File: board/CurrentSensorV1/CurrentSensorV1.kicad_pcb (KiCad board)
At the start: 2 copper layers, 40.8 x 24.2 mm, 19 parts, among them J1 USB_B_Micro, J2 FTDI_Header, J3 AudioJack3_GroundPinNumbers, J4 0, J5 0, J6 Conn_01x02_Female, J7 Conn_01x02_Female, SW2 SW_SPST_SM_DP, SW3 SW_SPST_SM_DP, U1 UA78M05CDCY, U2 ESP-01v090, U3 ADS1115

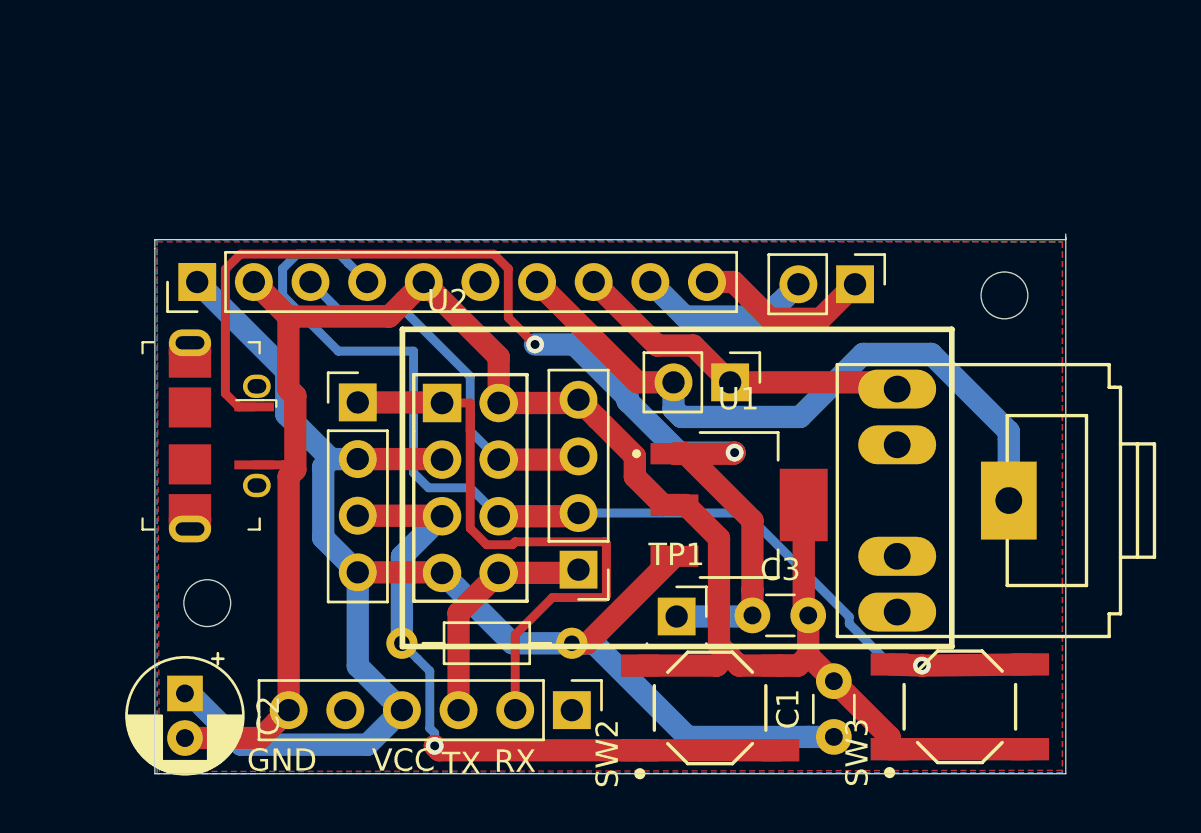
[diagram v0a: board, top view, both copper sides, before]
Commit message: Starting v4
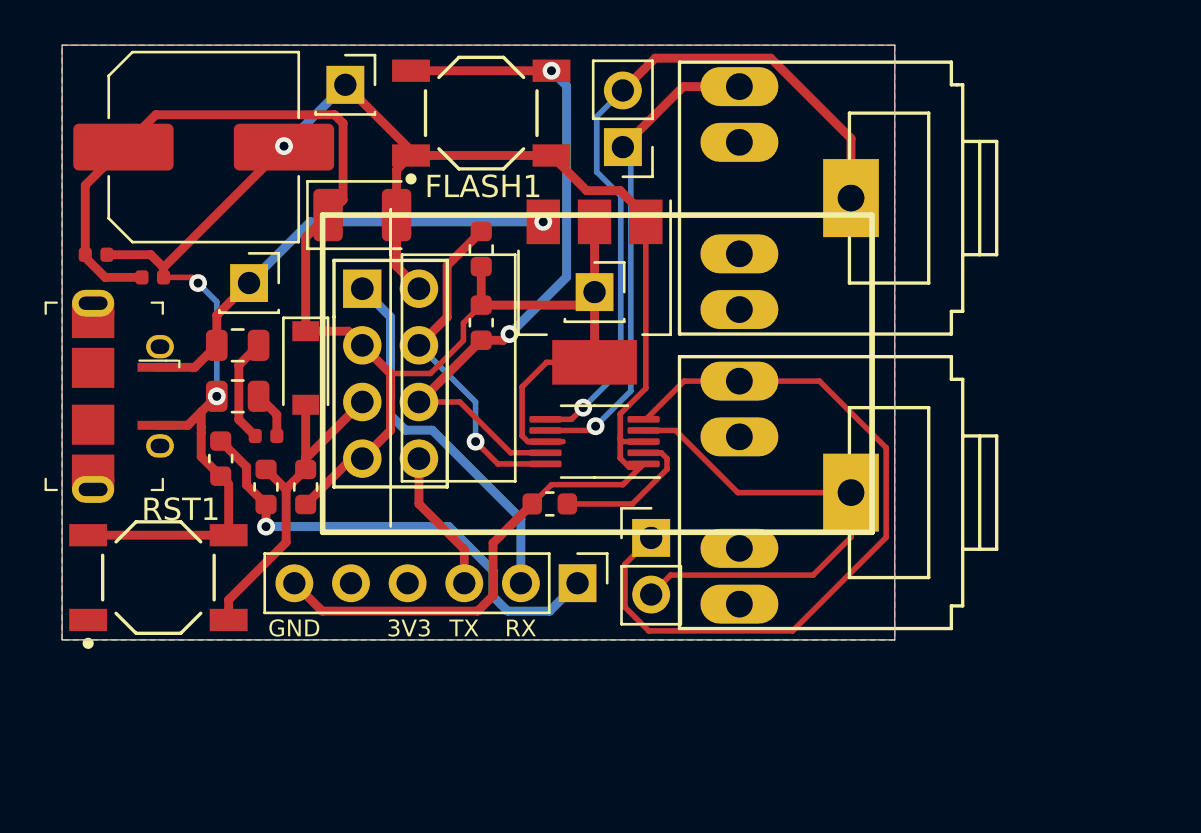
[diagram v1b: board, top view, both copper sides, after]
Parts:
- removed J4, J5: 0, Connector_PinHeader_2.54mm:PinHeader_1x04_P2.54mm_Vertical
- removed R4: R, Resistor_THT:R_Axial_DIN0204_L3.6mm_D1.6mm_P7.62mm_Horizontal
- removed REF** (x2): MountingHole_2.1mm, MountingHole:MountingHole_2.1mm
- added C4: 1000uF, Capacitor_SMD:C_Elec_8x10.2, F.Cu at (139.2, 69.8)
- added C5: 1uF, Capacitor_SMD:C_0402_1005Metric, F.Cu at (136.9, 75.7)
- added C6: 2.2uF, Capacitor_SMD:C_0603_1608Metric, F.Cu at (142.0, 85.1)
- added D1: D, Diode_SMD:D_SOD-123, F.Cu at (143.8, 79.8)
- added FB1: Ferrite_Bead, Resistor_SMD:R_0805_2012Metric, F.Cu at (140.7, 81.0)
- added FB2: Ferrite_Bead, Resistor_SMD:R_0805_2012Metric, F.Cu at (140.7, 78.7)
- added J8: AudioJack3_GroundPinNumbers, audio35mm:Tayda_3.5mm_stereo_TRS_jack_A-853, F.Cu at (166.6, 72.1)
- added R1: 10K, Resistor_SMD:R_0603_1608Metric, F.Cu at (151.6, 74.4)
- added R2: 10K, Resistor_SMD:R_0603_1608Metric, F.Cu at (151.6, 77.7)
- added R3: 10K, Resistor_SMD:R_0603_1608Metric, F.Cu at (154.7, 85.9)
- added R5: 680R, Resistor_SMD:R_0603_1608Metric, F.Cu at (140.0, 83.8)
- added R6: 10K, Resistor_SMD:R_0603_1608Metric, F.Cu at (143.8, 85.1)
- added TP2: TestPoint, Connector_PinSocket_2.54mm:PinSocket_1x01_P2.54mm_Vertical, F.Cu at (156.7, 76.4)
- added TP3: TestPoint, Connector_PinSocket_2.54mm:PinSocket_1x01_P2.54mm_Vertical, F.Cu at (145.5, 67.1)
- C1: value 0.1uF -> 1uF; footprint Capacitor_THT:C_Disc_D3.0mm_W1.6mm_P2.50mm -> Capacitor_SMD:C_0402_1005Metric
- C2: value 470uF -> 100uF; footprint Capacitor_THT:CP_Radial_D5.0mm_P2.00mm -> Capacitor_Tantalum_SMD:CP_EIA-3528-12_Kemet-T
- C3: value 0.33uF -> 1uF; footprint Capacitor_THT:C_Disc_D3.0mm_W1.6mm_P2.50mm -> Capacitor_SMD:C_0402_1005Metric
- TP1: value (none) -> TestPoint
- U1: value UA78M05CDCY -> ADS1015_IC; footprint UA78M05CDCY:SOT230P700X180-4N -> Package_SO:VSSOP-10_3x3mm_P0.5mm
- U3: value ADS1115 -> AMS1117-3.3; footprint Connector_PinHeader_2.54mm:PinHeader_1x10_P2.54mm_Vertical -> Package_TO_SOT_SMD:SOT-223-3_TabPin2
- moved FLASH1 34.2 mm to (151.6, 68.3)
- moved C3 33.6 mm to (134.4, 74.7)
- moved C1 28.8 mm to (142.0, 82.8), turned to 0 degrees
- moved RST1 25.4 mm to (137.2, 89.2)
- moved TP1 24.3 mm to (141.2, 75.9)
- moved C2 22.9 mm to (146.3, 72.9), turned to 0 degrees
- moved U3 17.8 mm to (156.7, 76.4), turned to 270 degrees
- moved J7 12.1 mm to (158.0, 69.8), turned to 180 degrees
- moved J6 7.82 mm to (159.3, 87.4), turned to 0 degrees
- moved J3 7.08 mm to (166.6, 85.3)
- moved U1 7.08 mm to (156.7, 83.1), turned to 180 degrees
- moved U2 6.25 mm to (146.3, 76.2)
- moved J2 5.70 mm to (156.0, 89.4)
- moved J1 4.69 mm to (136.9, 81.0)
- renumbered SW3 to FLASH1, SW2 to RST1
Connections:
- net Net-(J2-Pad2) renamed FTDI_RX
- net Net-(J2-Pad3) renamed FTDI_TX
- net Net-(J5-Pad3) renamed RST
- C1 pad 1: +3V3 -> Net-(C1-Pad1)
- C1 pad 2: GND -> Net-(C1-Pad2)
- C2 pad 2: GND -> ADDR
- C3 pad 1: VBUS -> +3V3
- C3 pad 2: GND -> ADDR
- FLASH1 pad 1: GND -> ADDR
- FLASH1 pad 2: GND -> ADDR
- J1 pad 5: GND -> ADDR
- J2 pad 6: GND -> ADDR
- J3 pad 1: Net-(J3-Pad1) -> AIN0
- J3 pad 3: Net-(J3-Pad3) -> AIN1
- J6 pad 1: Net-(J3-Pad3) -> AIN1
- J6 pad 2: Net-(J3-Pad1) -> AIN0
- J7 pad 1: Net-(J7-Pad1) -> AIN3
- J7 pad 2: Net-(J7-Pad2) -> AIN2
- RST1 pad 3: GND -> ADDR
- RST1 pad 4: GND -> ADDR
- U1 pad 1: VBUS -> ADDR
- U1 pad 2: GND -> /ALERT
- U1 pad 3: +3V3 -> ADDR
- U1 pad 4: GND -> AIN0
- U2 pad 2: GND -> ADDR
- U3 pad 1: +3V3 -> ADDR
- U3 pad 2: GND -> +3V3
- U3 pad 3: SCL -> VBUS
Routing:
- net ADDR: track 0.00 -> 96.3 mm, vias 0 -> 3
- net GND: track 90.6 -> 0.00 mm
- net AIN1: track 0.00 -> 34.3 mm
- net AIN2: track 0.00 -> 32.8 mm, vias 0 -> 1
- net Net-(J3-Pad1): track 30.1 -> 0.00 mm
- net VBUS: track 50.4 -> 22.3 mm, vias 2 -> 1
- net AIN0: track 0.00 -> 22.5 mm
- net AIN3: track 0.00 -> 22.0 mm, vias 0 -> 1
- net Net-(C6-Pad2): track 0.00 -> 21.4 mm, vias 0 -> 1
- net SDA: track 51.1 -> 31.4 mm, vias 1 -> 2
- net Net-(J3-Pad3): track 15.6 -> 0.00 mm
- net RST: track 31.0 -> 16.4 mm, vias 1 -> 0
- net FTDI_RX: track 27.7 -> 16.9 mm
- net Net-(J7-Pad1): track 7.97 -> 0.00 mm
- net Net-(J7-Pad2): track 7.88 -> 0.00 mm
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- added copper zone on F.Cu, net ADDR
- removed copper zone on F.Cu, net GND
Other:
- board size 40.8 x 24.2 mm -> 37.3 x 26.7 mm
